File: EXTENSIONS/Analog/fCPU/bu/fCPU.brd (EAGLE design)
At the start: 88 x 71 mm, 14 parts

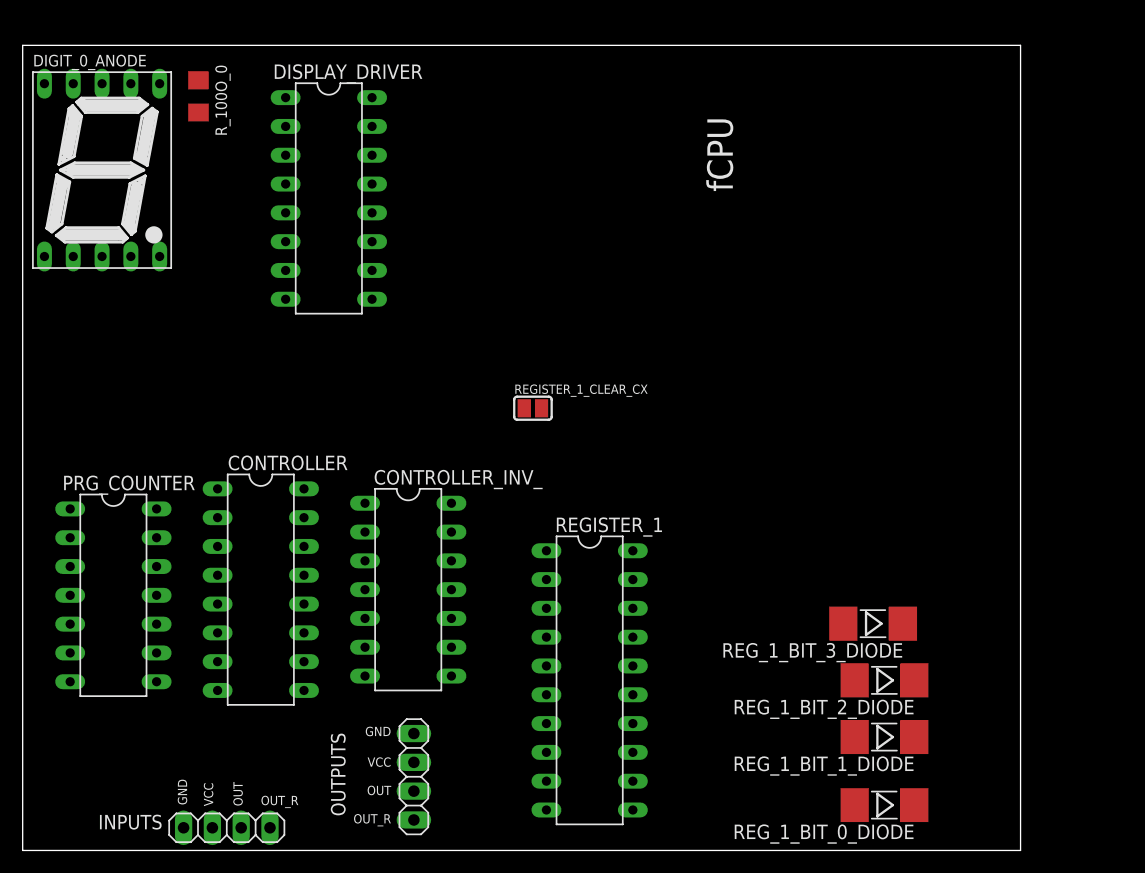
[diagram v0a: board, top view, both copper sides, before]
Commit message: Update fCPU
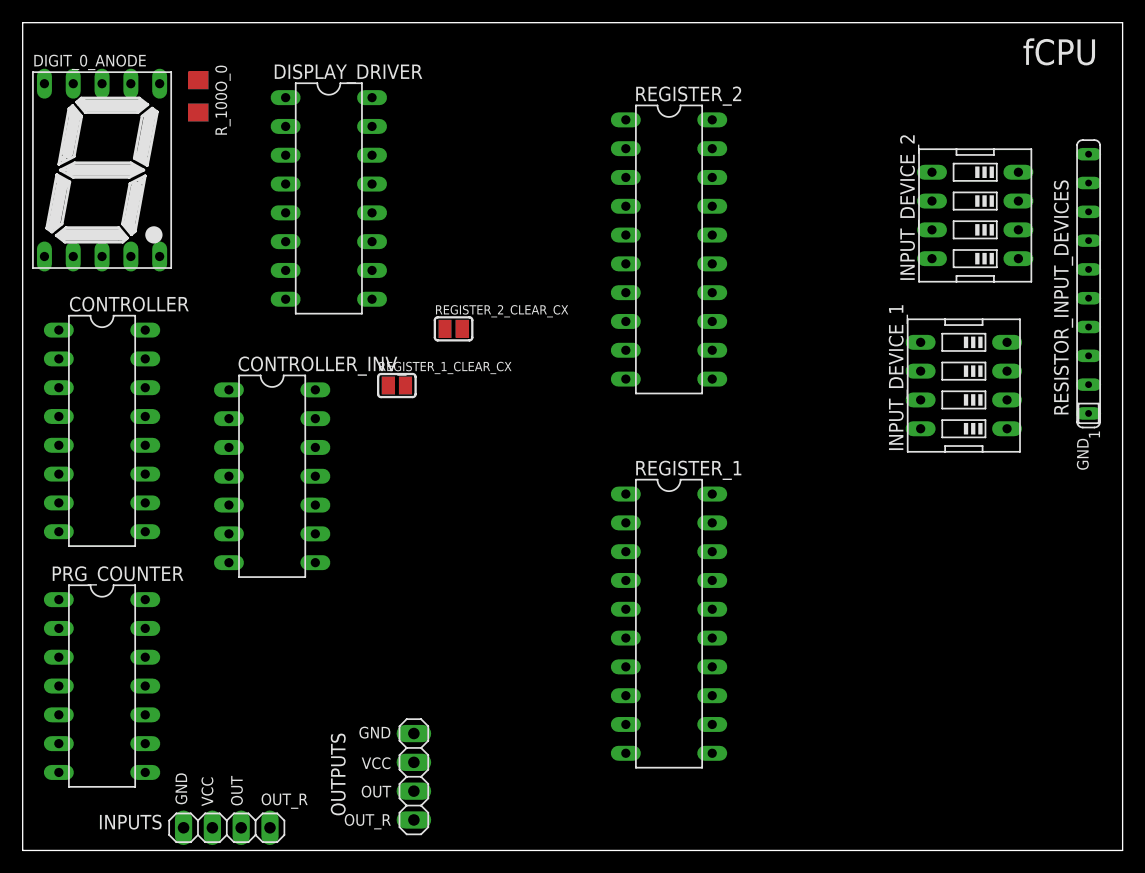
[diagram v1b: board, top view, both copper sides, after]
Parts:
- removed REG_1_BIT_0_DIODE, REG_1_BIT_1_DIODE, REG_1_BIT_2_DIODE, REG_1_BIT_3_DIODE: (no value), diode:MELF-MLL41
- added INPUT_DEVICE_1, INPUT_DEVICE_2: (no value), special:EDG-04
- added REGISTER_2: 74273N, 74xx-us:DIL20
- added REGISTER_2_CLEAR_CX: (no value), microbuilder:SOLDERJUMPER_REFLOW
- added RESISTOR_INPUT_DEVICES: (no value), resistor-sip:SIP10
- moved CONTROLLER 19.8 mm to (9.00, 49.0)
- moved CONTROLLER_INV_ 15.6 mm to (24.0, 45.0)
- moved REGISTER_1_CLEAR_CX 12.2 mm to (35.0, 53.0)
- moved REGISTER_1 8.60 mm to (59.0, 32.0)
- moved PRG_COUNTER 8.06 mm to (9.00, 26.5)
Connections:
- removed net N$2: REGISTER_1.2, REG_1_BIT_0_DIODE.A
- removed net N$3: REGISTER_1.5, REG_1_BIT_1_DIODE.A
- removed net N$4: REGISTER_1.6, REG_1_BIT_2_DIODE.A
- removed net N$5: REGISTER_1.9, REG_1_BIT_3_DIODE.A
- new net REGISTER_1_IN_BIT_0: INPUT_DEVICE_1.1, REGISTER_1.3, RESISTOR_INPUT_DEVICES.2
- new net REGISTER_1_IN_BIT_1: INPUT_DEVICE_1.2, REGISTER_1.4, RESISTOR_INPUT_DEVICES.3
- new net REGISTER_1_IN_BIT_2: INPUT_DEVICE_1.3, REGISTER_1.7, RESISTOR_INPUT_DEVICES.4
- new net REGISTER_1_IN_BIT_3: INPUT_DEVICE_1.4, REGISTER_1.8, RESISTOR_INPUT_DEVICES.5
- new net REGISTER_2_CLK: REGISTER_2.11
- new net REGISTER_2_CLR: REGISTER_2.1, REGISTER_2_CLEAR_CX.2
- new net REGISTER_2_IN_BIT_0: INPUT_DEVICE_2.1, REGISTER_2.3, RESISTOR_INPUT_DEVICES.6
- new net REGISTER_2_IN_BIT_1: INPUT_DEVICE_2.2, REGISTER_2.4, RESISTOR_INPUT_DEVICES.7
- new net REGISTER_2_IN_BIT_2: INPUT_DEVICE_2.3, REGISTER_2.7, RESISTOR_INPUT_DEVICES.8
- new net REGISTER_2_IN_BIT_3: INPUT_DEVICE_2.4, REGISTER_2.8, RESISTOR_INPUT_DEVICES.9
- net CTRL_OFF_2: now also REGISTER_2_CLEAR_CX.1
- net DTA_BUS_0: no longer REG_1_BIT_0_DIODE.C
- net DTA_BUS_1: no longer REG_1_BIT_1_DIODE.C
- net DTA_BUS_2: no longer REG_1_BIT_2_DIODE.C
- net DTA_BUS_3: no longer REG_1_BIT_3_DIODE.C
- net GND: now also REGISTER_1.13, REGISTER_1.14, REGISTER_1.17, REGISTER_1.18, REGISTER_2.10, REGISTER_2.13, REGISTER_2.14, REGISTER_2.17, REGISTER_2.18, RESISTOR_INPUT_DEVICES.1
- net VCC: now also INPUT_DEVICE_1.5, INPUT_DEVICE_1.6, INPUT_DEVICE_1.7, INPUT_DEVICE_1.8, INPUT_DEVICE_2.5, INPUT_DEVICE_2.6, INPUT_DEVICE_2.7, INPUT_DEVICE_2.8, REGISTER_2.20
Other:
- board size 88 x 71 mm -> 97 x 73 mm
